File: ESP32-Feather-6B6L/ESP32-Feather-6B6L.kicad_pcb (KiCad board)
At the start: 2 copper layers, 86.4 x 78.7 mm, 36 parts, among them J201 RJ45, J202 RJ45, J401 1 2 3 4 5 6 G, J501 + 1 2 3 4 5 6 -, U201 TCAN332DR, U301 LM2574N-5.0, U403 74HCT14, U501 TBD62084A

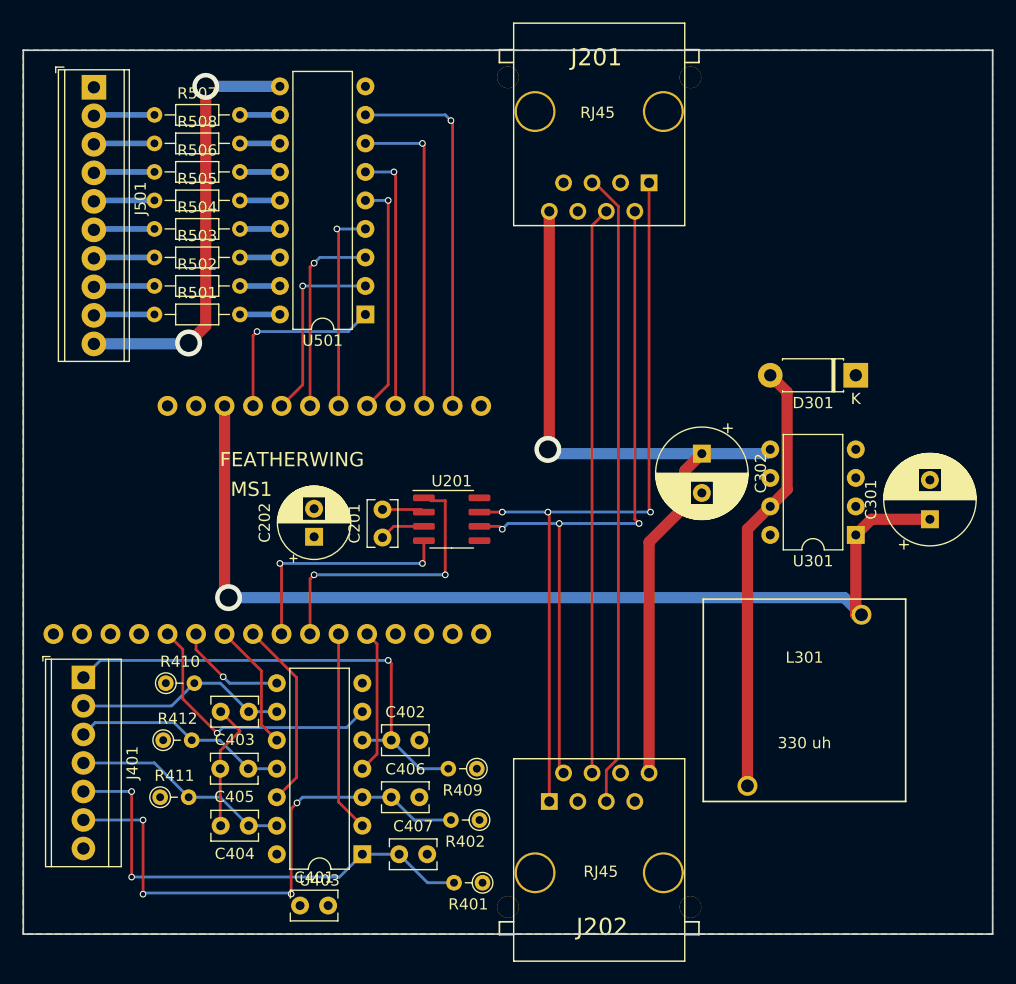
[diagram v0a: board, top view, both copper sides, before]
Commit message: Final through-hole tweaks.
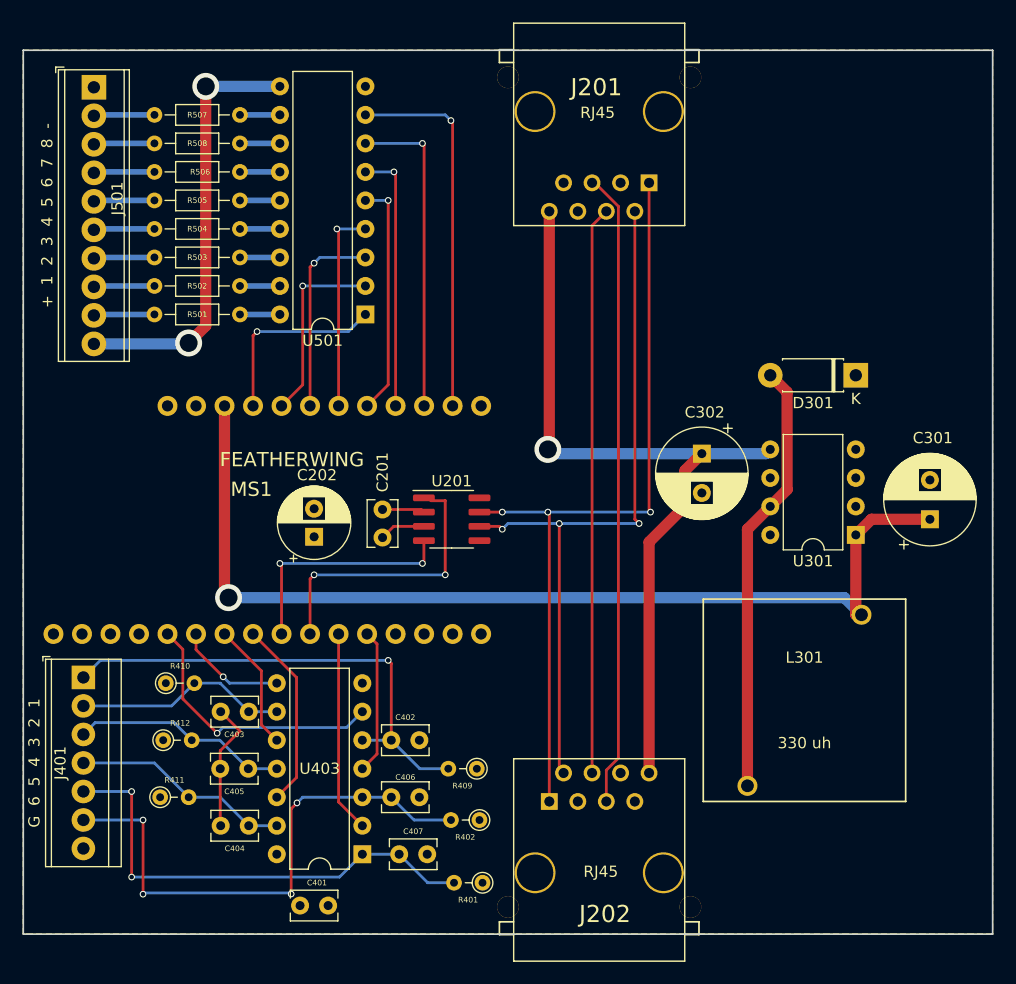
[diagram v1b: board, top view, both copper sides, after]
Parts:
- J401: value 1 2 3 4 5 6 G -> G 6 5 4 3 2 1
- J501: value + 1 2 3 4 5 6 - -> + 1 2 3 4 5 6 7 8 -
